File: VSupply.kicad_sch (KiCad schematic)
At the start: 12 parts, among them IC2 RAA2118054GP3#JA0

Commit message: updates to make better
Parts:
- D18: Manufacturer_Part_Number BZT52C3V3S -> MMSZ5233BS-7-F
- D19: Manufacturer_Part_Number BZT52C3V3S -> SZ4582
- D20: Manufacturer_Part_Number ULCE1005A015FR -> 0603ESDA-05N
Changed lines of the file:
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@@
 			)
 		)
-		(property "Manufacturer_Part_Number" "ULCE1005A015FR"
+		(property "Manufacturer_Part_Number" "0603ESDA-05N"
 			(at 120.65 64.77 0)
 			(effects
@@
 			)
 		)
-		(property "Manufacturer_Part_Number" "BZT52C3V3S"
+		(property "Manufacturer_Part_Number" "MMSZ5233BS-7-F"
 			(at 160.02 68.58 0)
 			(effects
@@
 			)
 		)
-		(property "Manufacturer_Part_Number" "BZT52C3V3S"
+		(property "Manufacturer_Part_Number" "SZ4582"
 			(at 45.72 66.04 0)
 			(effects

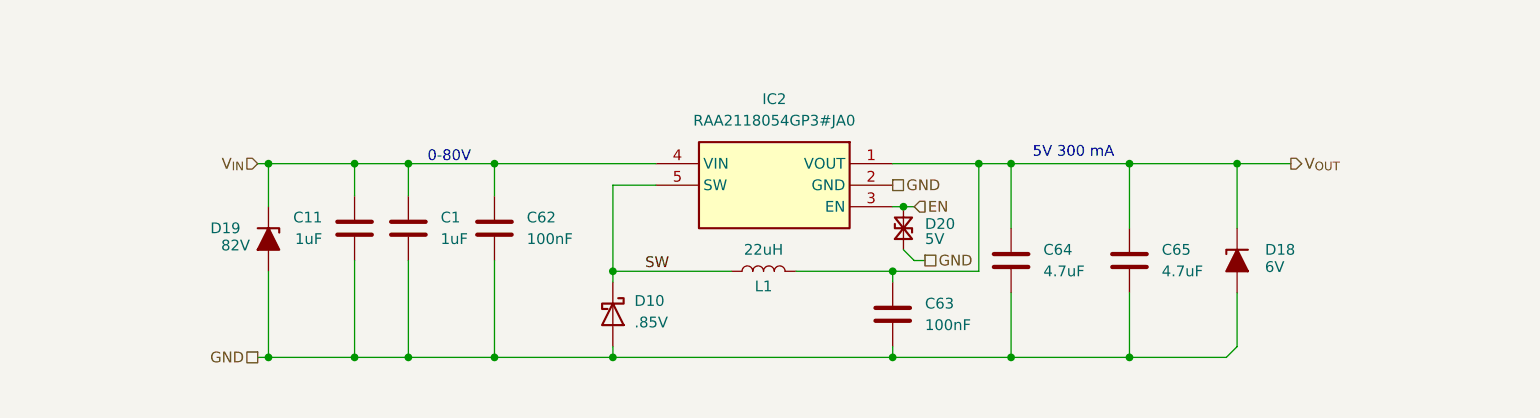
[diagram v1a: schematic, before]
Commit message: revision 2
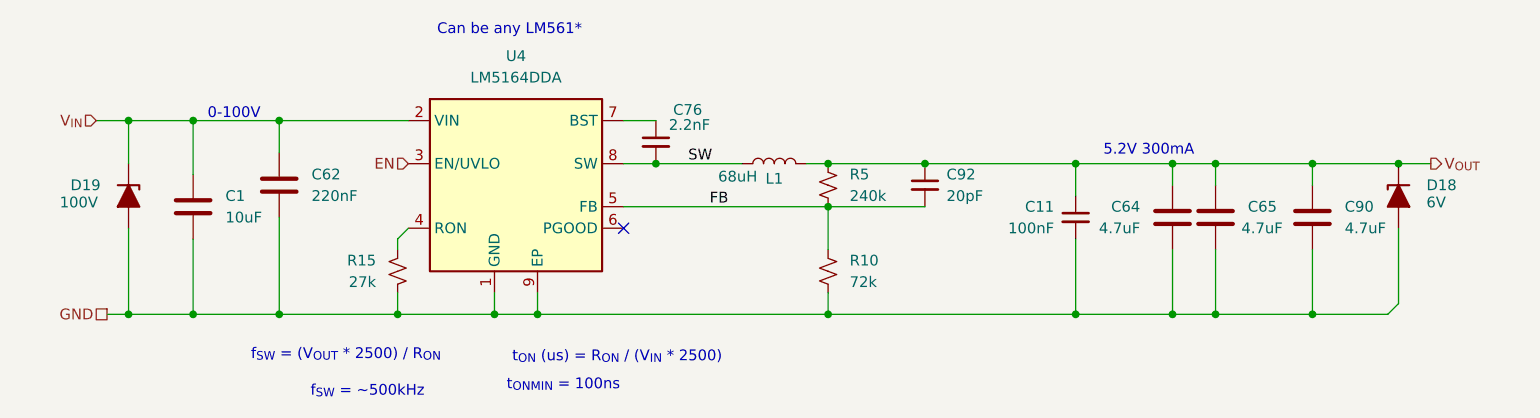
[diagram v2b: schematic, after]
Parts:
- removed C11: 1uF, Capacitor_SMD:C_0805_2012Metric, symbol Device:C
- removed C63: 100nF, Capacitor_SMD:C_0603_1608Metric, symbol Device:C
- removed D10: .85V, Diode_SMD:D_SOD-123, symbol Device:D_Schottky
- removed D20: 5V, Diode_SMD:D_0603_1608Metric, symbol Device:D_TVS_Small
- removed IC2: RAA2118054GP3#JA0, Package_TO_SOT_SMD:SOT-23-5, symbol RAA2118054GP3#JA0:RAA2118054GP3#JA0
- added C11: 100nF, Capacitor_SMD:C_0402_1005Metric, symbol Device:C_Small
- added C76: 2.2nF, Capacitor_SMD:C_0402_1005Metric, symbol Device:C_Small
- added C90: 4.7uF, Capacitor_SMD:C_0402_1005Metric, symbol Device:C
- added C92: 20pF, Capacitor_SMD:C_0402_1005Metric, symbol Device:C_Small
- added R10: 72k, Resistor_SMD:R_0402_1005Metric, symbol Device:R_Small_US
- added R15: 27k, Resistor_SMD:R_0402_1005Metric, symbol Device:R_Small_US
- added R5: 240k, Resistor_SMD:R_0402_1005Metric, symbol Device:R_Small_US
- added U4: LM5164DDA, Package_SO:HSOP-8-1EP_3.9x4.9mm_P1.27mm_EP2.41x3.1mm_ThermalVias, symbol Regulator_Switching:LM5164DDA
- C1: value 1uF -> 10uF; footprint Capacitor_SMD:C_0805_2012Metric -> Capacitor_SMD:C_1210_3225Metric; Manufacturer_Part_Number HHV0805R7105K101NSLJ -> FS32X475K101EGG
- C62: value 100nF -> 220nF
- C64, C65: footprint Capacitor_SMD:C_0603_1608Metric -> Capacitor_SMD:C_0402_1005Metric
- D18: footprint Diode_SMD:D_SOD-323 -> Diode_SMD:D_SOD-882
- D19: value 82V -> 100V; footprint Diode_SMD:D_SMA -> Diode_SMD:D_SOD-123F
- L1: value 22uH -> 68uH; footprint Inductor_SMD:L_Abracon_ASPI-3012S -> Inductor_SMD:L_Abracon_ASPI-4030S
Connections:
- net EN: now also U4.3 (EN/UVLO)
- net GND: now also C11.2, C90.2, R10.2, R15.2, U4.1 (GND), U4.9 (EP)
- net SW: now also C76.2, U4.8 (SW)
- net V_{IN}: now also U4.2 (VIN)
- net V_{OUT}: now also C11.1, C90.1, C92.1, R5.1
- new net: C76.1, U4.7 (BST)
- new net: R15.1, U4.4 (RON)
- new net FB: C92.2, R10.1, R5.2, U4.5 (FB)
- no-connect marks 0 -> 1
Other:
- note added: "0-100V"
- note added: "5.2V 300mA"
- note added: "Can be any LM561*"
- note added: "f_{SW} = (V_{OUT} * 2500) / R_{ON}"
- note added: "f_{SW} = ~500kHz"
- note added: "t_{ONMIN} = 100ns"
- note added: "t_{ON} (us) = R_{ON} / (V_{IN} * 2500)"
- note removed: "0-80V"
- note removed: "5V 300 mA"
- moved on the sheet: C62, C64, C65, D18, D19, L1
